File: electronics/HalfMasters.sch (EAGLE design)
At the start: 17 parts, among them J1 F-1X04-SIP-100-40, U1 RASPBERRY_PICOSMD-TH, U2 L7805CV

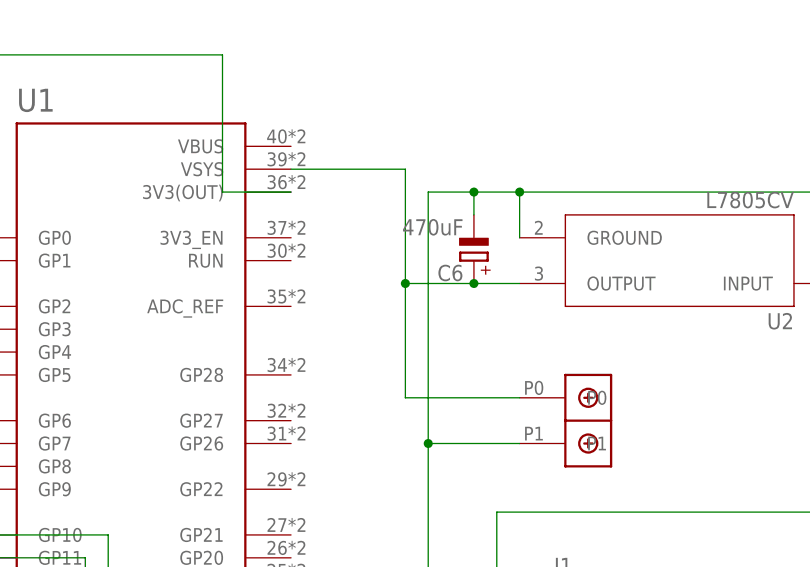
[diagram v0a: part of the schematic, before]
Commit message: refacotr: code upload to github
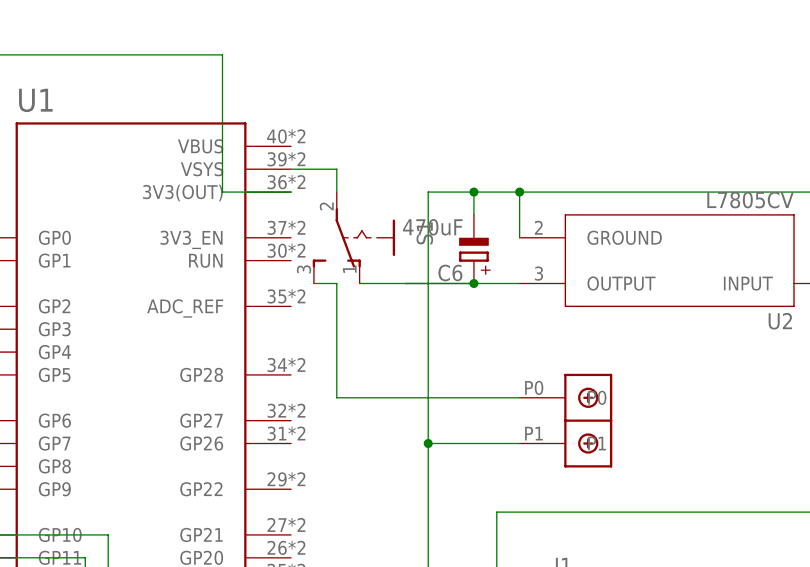
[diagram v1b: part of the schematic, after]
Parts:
- added S1: (no value), switch:255SB
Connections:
- new net N$3: S1.S, U$5.P0
- new net N$7: S1.P, U1.VSYS
- net N$18: now also S1.O; no longer U$5.P0, U1.VSYS
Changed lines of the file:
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@@
 <part name="U$5" library="Terminal Block Connector" deviceset="DBCONN-1X2" device=""/>
 <part name="J1" library="con-headers-jp" deviceset="F-1X04-" device="SIP-100-40"/>
+<part name="S1" library="switch" library_urn="urn:adsk.eagle:library:380" deviceset="255SB" device="" package3d_urn="urn:adsk.eagle:package:27679/1"/>
 </parts>
 <sheets>
@@
 <attribute name="NAME" x="105.41" y="31.242" size="1.778" layer="95"/>
 </instance>
+<instance part="S1" gate="1" x="83.82" y="68.58" smashed="yes" rot="R180">
+<attribute name="NAME" x="90.17" y="70.485" size="1.778" layer="95" rot="R270"/>
+<attribute name="VALUE" x="87.63" y="65.405" size="1.778" layer="96" rot="R270"/>
+</instance>
 </instances>
 <busses>
@@
 <net name="N$18" class="0">
 <segment>
-<pinref part="U1" gate="U$1" pin="VSYS"/>
-<wire x1="76.2" y1="76.2" x2="88.9" y2="76.2" width="0.1524" layer="91"/>
-<wire x1="88.9" y1="76.2" x2="88.9" y2="63.5" width="0.1524" layer="91"/>
 <pinref part="U2" gate="G$1" pin="OUTPUT"/>
 <wire x1="88.9" y1="63.5" x2="96.52" y2="63.5" width="0.1524" layer="91"/>
@@
 <wire x1="96.52" y1="63.5" x2="101.6" y2="63.5" width="0.1524" layer="91"/>
 <junction x="96.52" y="63.5"/>
-<pinref part="U$5" gate="G$1" pin="P0"/>
-<wire x1="88.9" y1="63.5" x2="88.9" y2="50.8" width="0.1524" layer="91"/>
-<wire x1="88.9" y1="50.8" x2="101.6" y2="50.8" width="0.1524" layer="91"/>
-<junction x="88.9" y="63.5"/>
+<pinref part="S1" gate="1" pin="O"/>
+<wire x1="83.82" y1="63.5" x2="96.52" y2="63.5" width="0.1524" layer="91"/>
 </segment>
 </net>
@@
 </segment>
 </net>
+<net name="N$3" class="0">
+<segment>
+<pinref part="U$5" gate="G$1" pin="P0"/>
+<wire x1="81.28" y1="50.8" x2="101.6" y2="50.8" width="0.1524" layer="91"/>
+<pinref part="S1" gate="1" pin="S"/>
+<wire x1="78.74" y1="63.5" x2="81.28" y2="63.5" width="0.1524" layer="91"/>
+<wire x1="81.28" y1="63.5" x2="81.28" y2="50.8" width="0.1524" layer="91"/>
+</segment>
+</net>
+<net name="N$7" class="0">
+<segment>
+<pinref part="S1" gate="1" pin="P"/>
+<pinref part="U1" gate="U$1" pin="VSYS"/>
+<wire x1="81.28" y1="73.66" x2="81.28" y2="76.2" width="0.1524" layer="91"/>
+<wire x1="81.28" y1="76.2" x2="76.2" y2="76.2" width="0.1524" layer="91"/>
+</segment>
+</net>
